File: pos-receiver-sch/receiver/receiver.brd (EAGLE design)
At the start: 26 x 21.9 mm, 15 parts, among them IC1 AD8599R

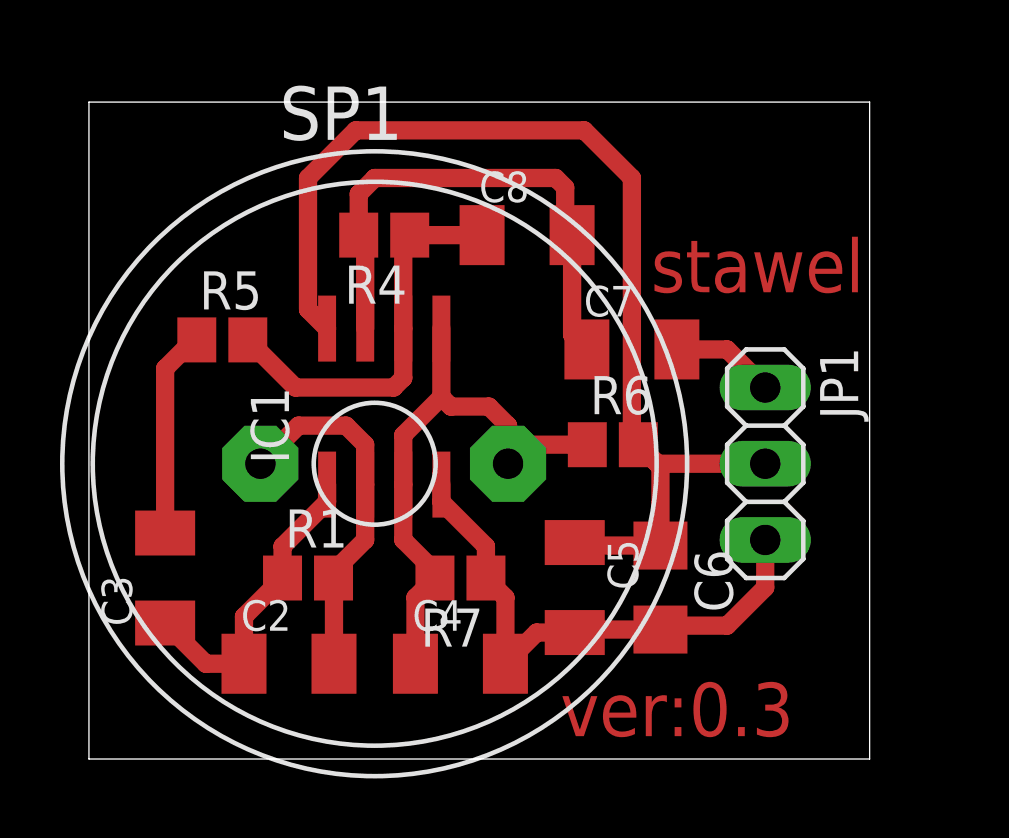
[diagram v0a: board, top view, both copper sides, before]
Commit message: pcb
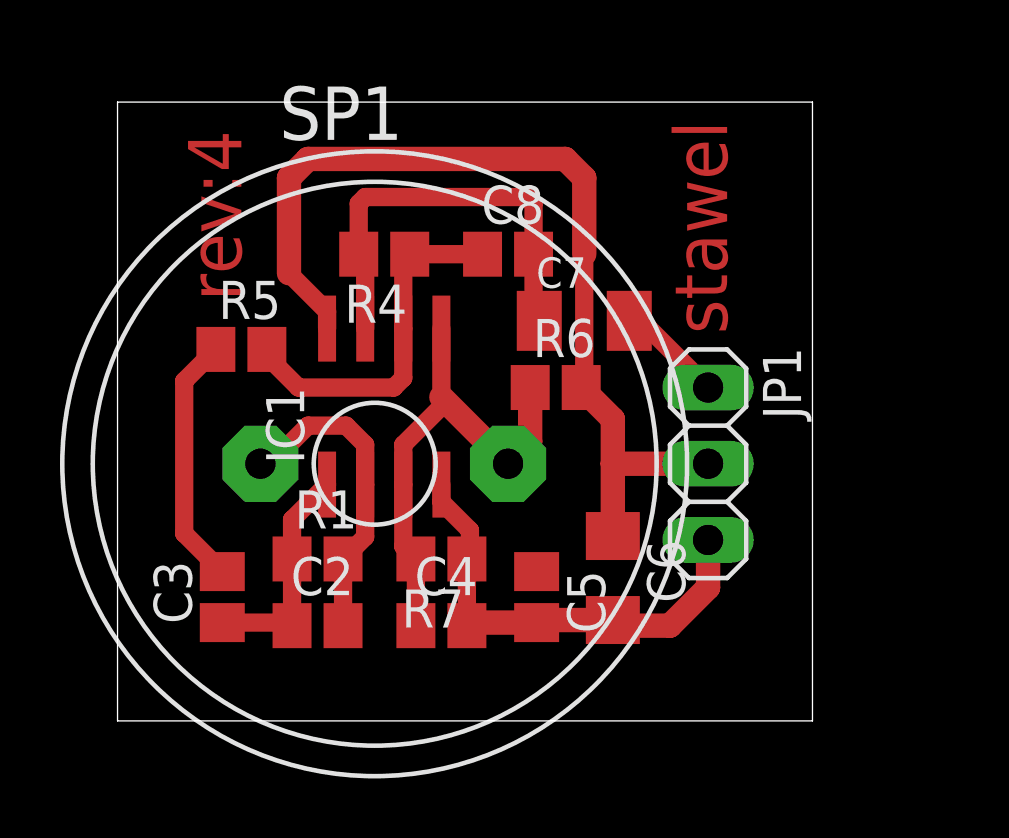
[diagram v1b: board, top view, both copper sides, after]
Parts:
- C2: value 100p -> 12p; device resistor:C1206K -> resistor:C0805
- C3, C4, C5, C8: device resistor:C1206K -> resistor:C0805
- IC1: value AD8599R -> NE5532D; device analog-devices:SO8 -> linear:SO08
- R1: value 33k -> 1M
- moved R6 2.69 mm to (40.0, 29.8)
- moved C3 2.01 mm to (28.9, 22.9)
- moved JP1 1.91 mm to (45.1, 27.3)
- moved C7 1.85 mm to (41.0, 32.1)
- moved C6 1.62 mm to (41.9, 23.5)
- moved C2 1.59 mm to (32.1, 21.9)
- moved C4 1.42 mm to (36.2, 21.9)
- moved C5 1.31 mm to (39.4, 22.9)
- moved C8 0.90 mm to (38.4, 34.3)
- moved R7 0.90 mm to (36.2, 24.1)
- moved R5 0.71 mm to (29.5, 31.1)
- moved R1 0.71 mm to (32.1, 24.1)
- moved R4 0.63 mm to (34.3, 34.3)
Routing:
- net VCC: track 37.4 -> 31.6 mm
- net N$5: track 17.5 -> 14.3 mm
- net N$8: track 10.3 -> 7.55 mm
- net GND: track 18.2 -> 15.5 mm
- net N$9: track 19.2 -> 16.6 mm
- net N$6: track 6.93 -> 8.37 mm
- net N$3: track 12.0 -> 10.6 mm
- net N$4: track 13.2 -> 12.0 mm
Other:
- board size 26 x 21.9 mm -> 23.2 x 20.6 mm
- board text added: "rev:4"
- board text removed: "ver:0.3"
